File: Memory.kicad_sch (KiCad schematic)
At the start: 8 parts, among them IC1 NAND_MT29F1G08ABAEAWP-IT_E_TR, IC2 SRAM_R1LP5256ESA-5SI#S1_TSOP28

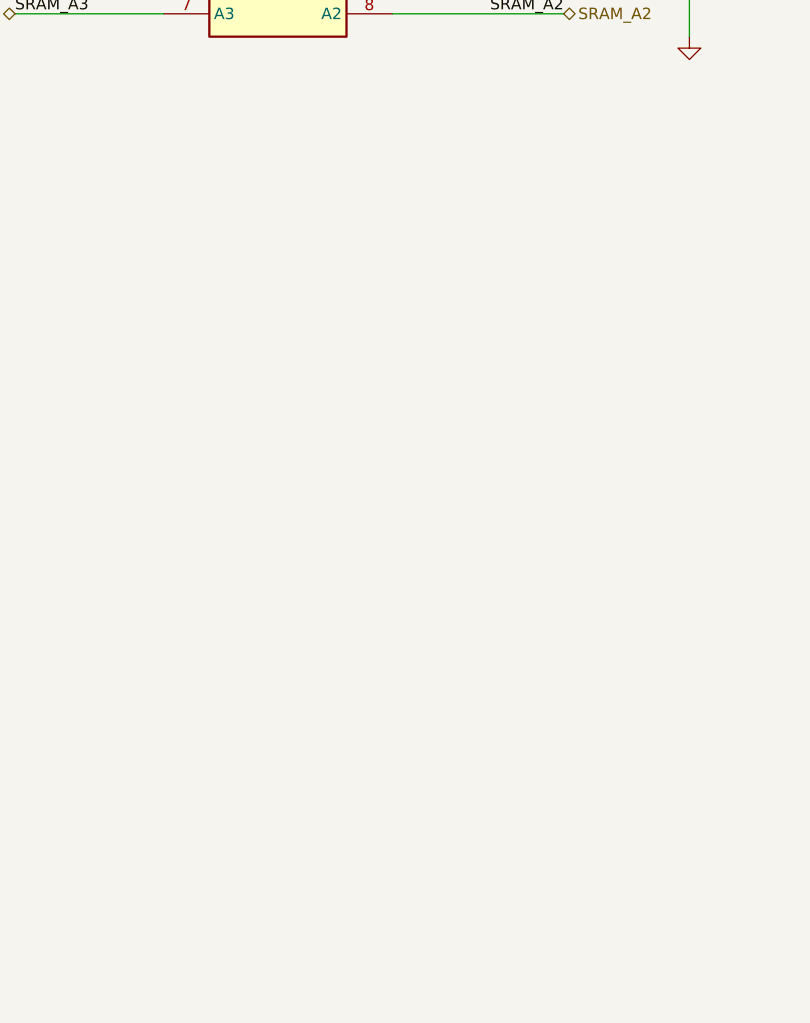
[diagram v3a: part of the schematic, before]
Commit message: Update
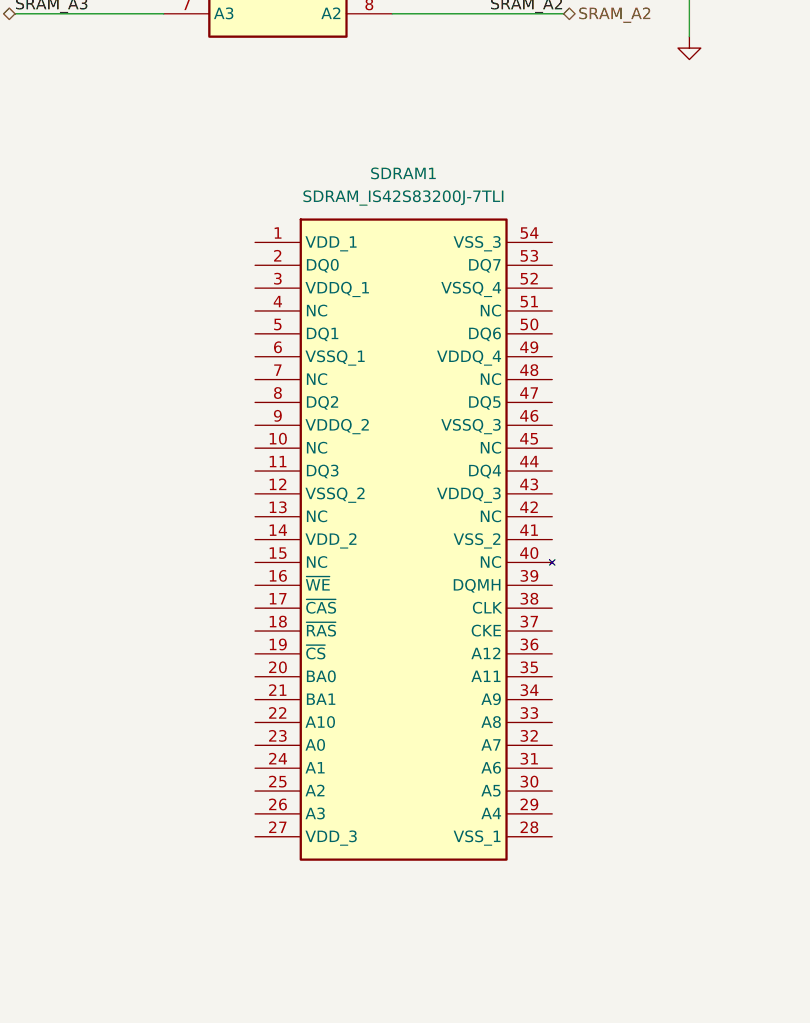
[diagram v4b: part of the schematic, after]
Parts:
- added SDRAM1: SDRAM_IS42S83200J-7TLI, Personal_Project:SDRAM_IS42S16320F-6TL, symbol Personal_Projects:SDRAM_IS42S83200J-7TLI
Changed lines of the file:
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@@
+	)
+	(symbol
+		(lib_id "Personal_Projects:SDRAM_IS42S83200J-7TLI")
+		(at 135.89 171.45 0)
+		(unit 1)
+		(exclude_from_sim no)
+		(in_bom yes)
+		(on_board yes)
+		(dnp no)
+		(fields_autoplaced yes)
+		(property "Reference" "SDRAM1"
+			(at 152.4 163.83 0)
+			(effects
+				(font
+					(size 1.27 1.27)
+				)
+			)
+		)
+		(property "Value" "SDRAM_IS42S83200J-7TLI"
+			(at 152.4 166.37 0)
+			(effects
+				(font
+					(size 1.27 1.27)
+				)
+			)
+		)
+		(property "Footprint" "Personal_Project:SDRAM_IS42S16320F-6TL"
+			(at 165.1 266.37 0)
+			(effects
+				(font
+					(size 1.27 1.27)
+				)
+				(justify left top)
+				(hide yes)
+			)
+		)
+		(property "Datasheet" "http://www.issi.com/WW/pdf/42-45R-S_86400F-16320F.pdf"
+			(at 165.1 366.37 0)
+			(effects
+				(font
+					(size 1.27 1.27)
+				)
+				(justify left top)
+				(hide yes)
+			)
+		)
+		(property "Description" "DRAM 512M, 3.3V, SDRAM, 32Mx16, 166MHz, 54 pin TSOP II (400 mil) RoHS"
+			(at 135.89 165.1 0)
+			(effects
+				(font
+					(size 1.27 1.27)
+				)
+				(hide yes)
+			)
+		)
+		(property "Height" "1.2"
+			(at 165.1 566.37 0)
+			(effects
+				(font
+					(size 1.27 1.27)
+				)
+				(justify left top)
+				(hide yes)
+			)
+		)
+		(property "Mouser Part Number" "870-42S16320F6TL"
+			(at 165.1 666.37 0)
+			(effects
+				(font
+					(size 1.27 1.27)
+				)
+				(justify left top)
+				(hide yes)
+			)
+		)
+		(property "Mouser Price/Stock" "https://www.mouser.co.uk/ProductDetail/ISSI/IS42S16320F-6TL?qs=N2Tevpb%252BvoZt27KFhoNVKQ%3D%3D"
+			(at 165.1 766.37 0)
+			(effects
+				(font
+					(size 1.27 1.27)
+				)
+				(justify left top)
+				(hide yes)
+			)
+		)
+		(property "Manufacturer_Name" "Integrated Silicon Solution Inc."
+			(at 165.1 866.37 0)
+			(effects
+				(font
+					(size 1.27 1.27)
+				)
+				(justify left top)
+				(hide yes)
+			)
+		)
+		(property "Manufacturer_Part_Number" "IS42S16320F-6TL"
+			(at 165.1 966.37 0)
+			(effects
+				(font
+					(size 1.27 1.27)
+				)
+				(justify left top)
+				(hide yes)
+			)
+		)
+		(pin "33"
+		)
+		(pin "34"
+		)
+		(pin "31"
+		)
+		(pin "32"
+		)
+		(pin "24"
+		)
+		(pin "25"
+		)
+		(pin "41"
+		)
+		(pin "42"
+		)
+		(pin "43"
+		)
+		(pin "5"
+		)
+		(pin "50"
+		)
+		(pin "51"
+		)
+		(pin "52"
+		)
+		(pin "53"
+		)
+		(pin "54"
+		)
+		(pin "6"
+		)
+		(pin "7"
+		)
+		(pin "8"
+		)
+		(pin "9"
+		)
+		(pin "1"
+		)
+		(pin "10"
+		)
+		(pin "19"
+		)
+		(pin "2"
+		)
+		(pin "17"
+		)
+		(pin "18"
+		)
+		(pin "37"
+		)
+		(pin "38"
+		)
+		(pin "35"
+		)
+		(pin "36"
+		)
+		(pin "26"
+		)
+		(pin "27"
+		)
+		(pin "47"
+		)
+		(pin "48"
+		)
+		(pin "49"
+		)
+		(pin "4"
+		)
+		(pin "13"
+		)
+		(pin "14"
+		)
+		(pin "28"
+		)
+		(pin "29"
+		)
+		(pin "15"
+		)
+		(pin "16"
+		)
+		(pin "12"
+		)
+		(pin "20"
+		)
+		(pin "21"
+		)
+		(pin "3"
+		)
+		(pin "30"
+		)
+		(pin "22"
+		)
+		(pin "23"
+		)
+		(pin "44"
+		)
+		(pin "45"
+		)
+		(pin "46"
+		)
+		(pin "11"
+		)
+		(pin "39"
+		)
+		(pin "40"
+		)
+		(instances
+			(project ""
+				(path "/9b48e30a-b912-4658-a133-1a15707d5b7d/c1273a5b-dc13-48da-a35d-ed40e44ccc48"
+					(reference "SDRAM1")
+					(unit 1)
+				)
+			)
+		)
 	)
 	(symbol

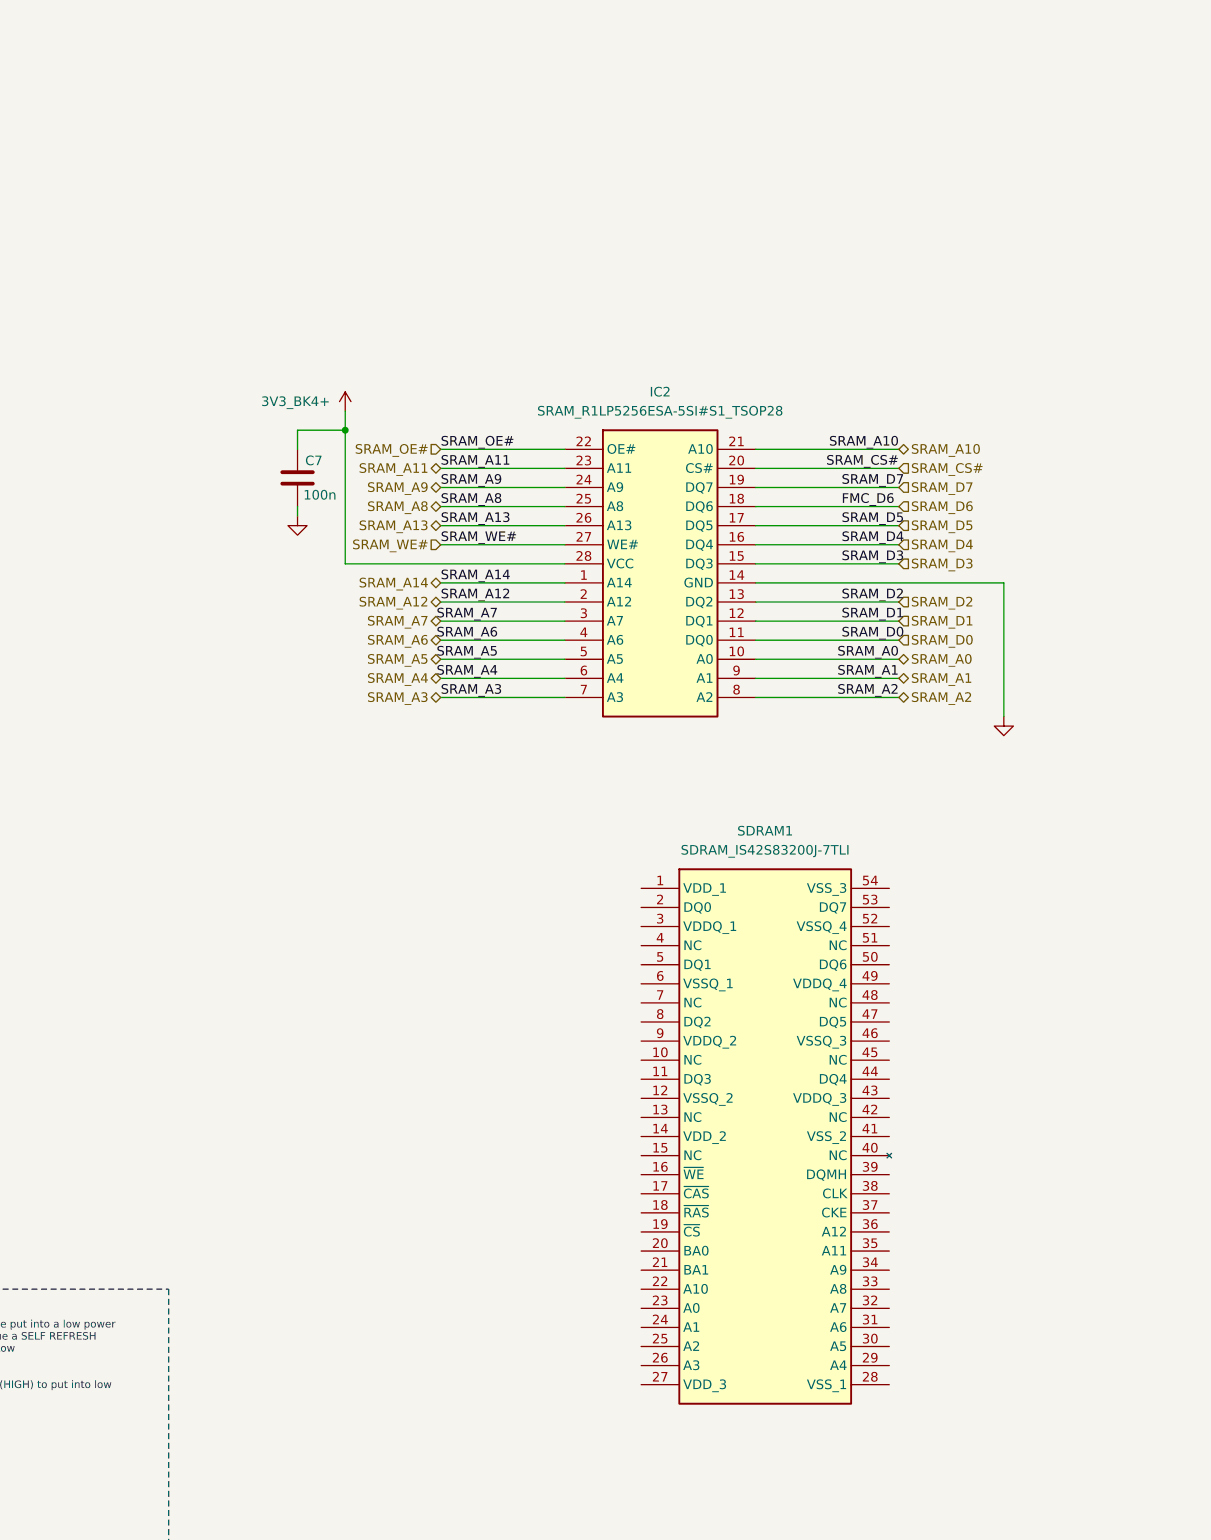
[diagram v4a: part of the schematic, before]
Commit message: Update
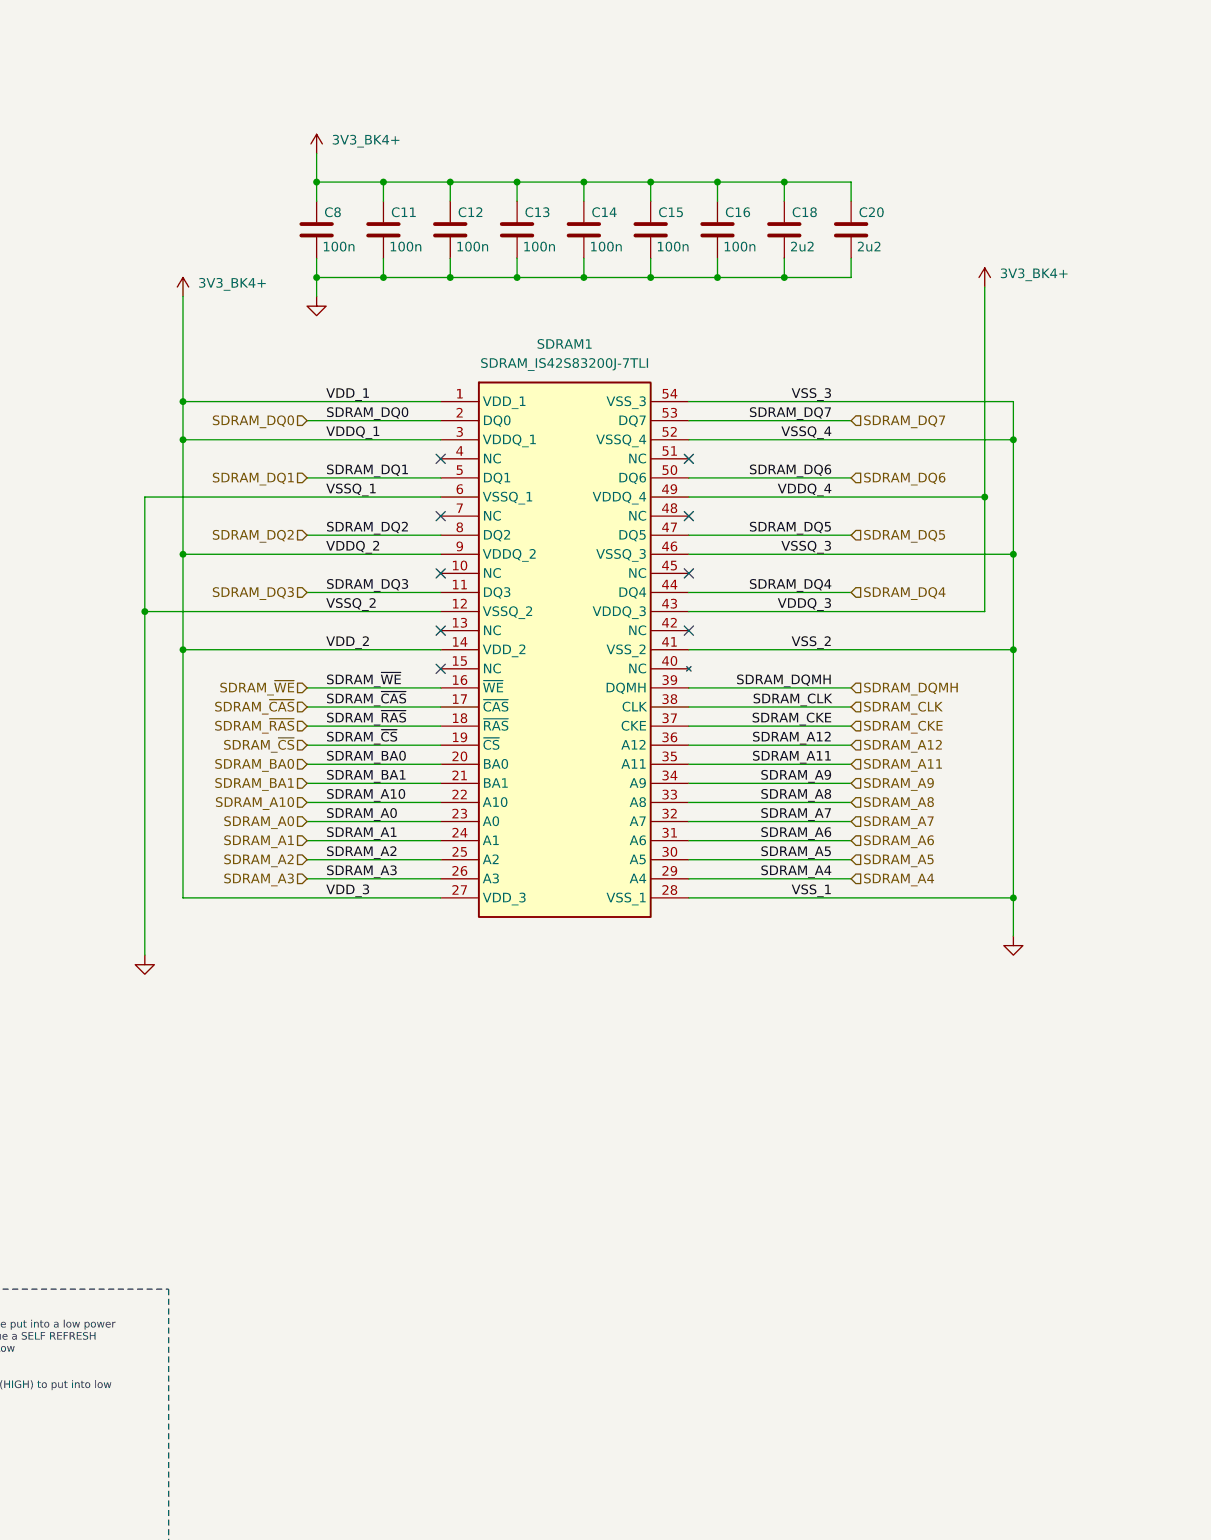
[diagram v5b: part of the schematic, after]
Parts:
- removed C7: 100n, Capacitor_SMD:C_0603_1608Metric, symbol Device:C
- removed IC2: SRAM_R1LP5256ESA-5SI#S1_TSOP28, Personal_Project:SRAM_R1LV5256ESA5SIS1_TSOP28, symbol Personal_Projects:SRAM_R1LP5256ESA-5SI#S1_TSOP28
- added C11, C12, C13, C14, C15, C16, C8: 100n, Capacitor_SMD:C_0603_1608Metric, symbol Device:C
- added C18, C20: 2u2, Capacitor_SMD:C_0603_1608Metric, symbol Device:C
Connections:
- net 3V3_BK4+: now also SDRAM1.1 (VDD_1), SDRAM1.14 (VDD_2), SDRAM1.27 (VDD_3), SDRAM1.3 (VDDQ_1), SDRAM1.43 (VDDQ_3), SDRAM1.49 (VDDQ_4), SDRAM1.9 (VDDQ_2), C11.1, C12.1, C13.1, C14.1, C15.1, C16.1, C18.1, C20.1, C8.1
- net GND: now also SDRAM1.12 (VSSQ_2), SDRAM1.28 (VSS_1), SDRAM1.41 (VSS_2), SDRAM1.46 (VSSQ_3), SDRAM1.52 (VSSQ_4), SDRAM1.54 (VSS_3), SDRAM1.6 (VSSQ_1), C11.2, C12.2, C13.2, C14.2, C15.2, C16.2, C18.2, C20.2, C8.2
- net SDRAM_DQ3: now reaches SDRAM1.11 (DQ3)
- net SDRAM_~{WE}: now reaches SDRAM1.16 (~{WE})
- net SDRAM_~{CAS}: now reaches SDRAM1.17 (~{CAS})
- net SDRAM_~{RAS}: now reaches SDRAM1.18 (~{RAS})
- net SDRAM_~{CS}: now reaches SDRAM1.19 (~{CS})
- net SDRAM_DQ0: now reaches SDRAM1.2 (DQ0)
- net SDRAM_BA0: now reaches SDRAM1.20 (BA0)
- net SDRAM_BA1: now reaches SDRAM1.21 (BA1)
- net SDRAM_A10: now reaches SDRAM1.22 (A10)
- net SDRAM_A0: now reaches SDRAM1.23 (A0)
- net SDRAM_A1: now reaches SDRAM1.24 (A1)
- net SDRAM_A2: now reaches SDRAM1.25 (A2)
- net SDRAM_A3: now reaches SDRAM1.26 (A3)
- net SDRAM_A4: now reaches SDRAM1.29 (A4)
- net SDRAM_A5: now reaches SDRAM1.30 (A5)
- net SDRAM_A6: now reaches SDRAM1.31 (A6)
- net SDRAM_A7: now reaches SDRAM1.32 (A7)
- net SDRAM_A8: now reaches SDRAM1.33 (A8)
- net SDRAM_A9: now reaches SDRAM1.34 (A9)
- net SDRAM_A11: now reaches SDRAM1.35 (A11)
- net SDRAM_A12: now reaches SDRAM1.36 (A12)
- net SDRAM_CKE: now reaches SDRAM1.37 (CKE)
- net SDRAM_CLK: now reaches SDRAM1.38 (CLK)
- net SDRAM_DQMH: now reaches SDRAM1.39 (DQMH)
- net SDRAM_DQ4: now reaches SDRAM1.44 (DQ4)
- net SDRAM_DQ5: now reaches SDRAM1.47 (DQ5)
- net SDRAM_DQ1: now reaches SDRAM1.5 (DQ1)
- net SDRAM_DQ6: now reaches SDRAM1.50 (DQ6)
- net SDRAM_DQ7: now reaches SDRAM1.53 (DQ7)
- net SDRAM_DQ2: now reaches SDRAM1.8 (DQ2)
- no-connect marks 25 -> 34
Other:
- moved on the sheet: SDRAM1
